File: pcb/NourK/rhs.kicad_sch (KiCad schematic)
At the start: 1 part

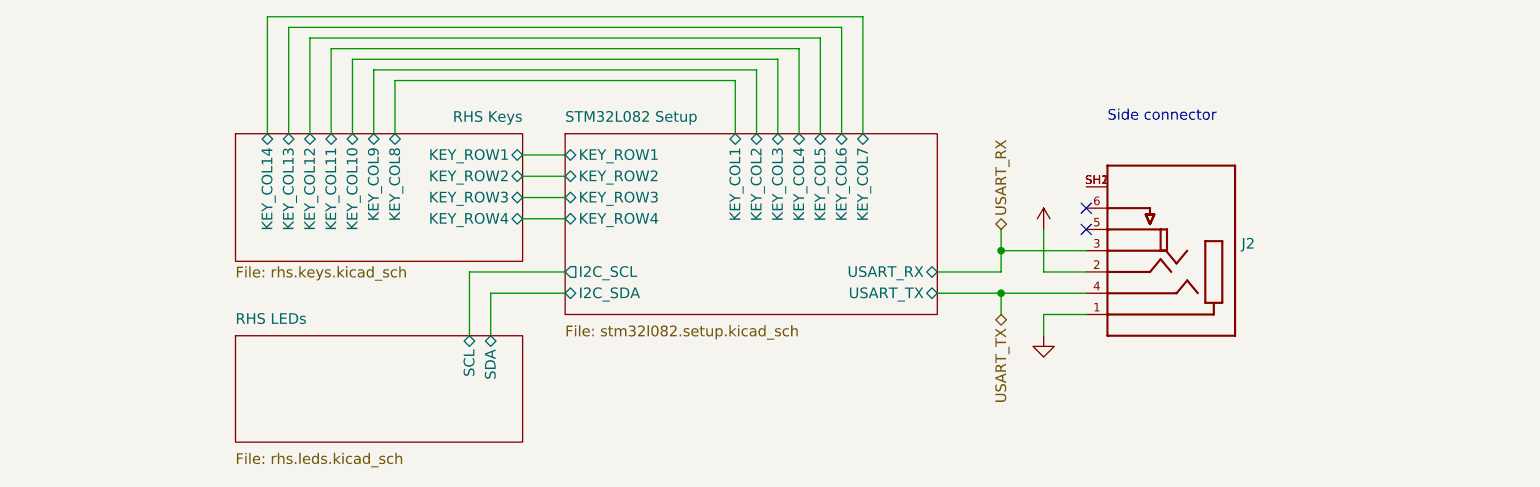
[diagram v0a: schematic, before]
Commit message: Draft LHS tracks
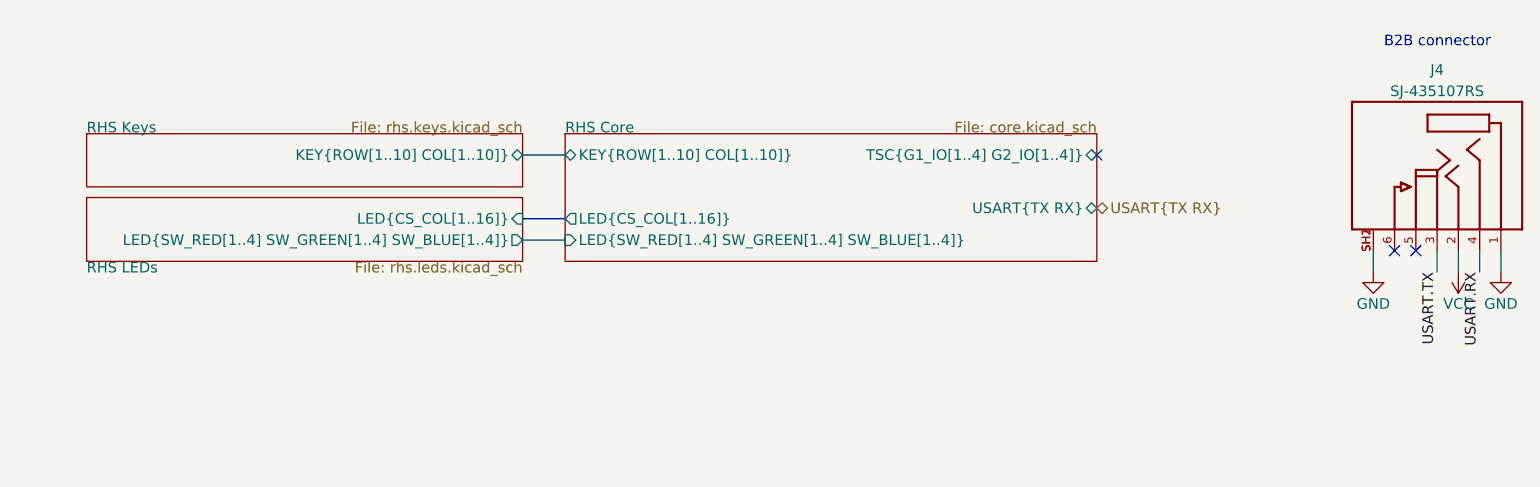
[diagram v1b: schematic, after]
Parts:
- removed J2: (no value), symbol Nour_KB:SJ-435107RS
- added J4: SJ-435107RS, Nour_KB:CUI_SJ-435107RS, symbol Nour_KB:SJ-435107RS
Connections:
- net GND: now also J4.1, J4.SH1, J4.SH2
- net VCC: now also J4.2
- new net USART.RX: J4.4
- new net USART.TX: J4.3
- no-connect marks 2 -> 3
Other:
- removed sheet STM32L082 Setup
- added sheet RHS Core (core.kicad_sch)
- sheet RHS Keys ports: added KEY{ROW[1..10] COL[1..10]}; removed KEY_COL10, KEY_COL11, KEY_COL12, KEY_COL13, KEY_COL14, KEY_COL8, KEY_COL9, KEY_ROW1, KEY_ROW2, KEY_ROW3, KEY_ROW4
- sheet RHS LEDs ports: added LED{CS_COL[1..16]}, LED{SW_RED[1..4] SW_GREEN[1..4] SW_BLUE[1..4]}; removed SCL, SDA
- note added: "B2B connector"
- note removed: "Side connector"
